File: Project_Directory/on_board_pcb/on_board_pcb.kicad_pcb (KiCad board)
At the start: 2 copper layers, 129.5 x 54.5 mm, 10 parts, among them U1 Teensy4.1

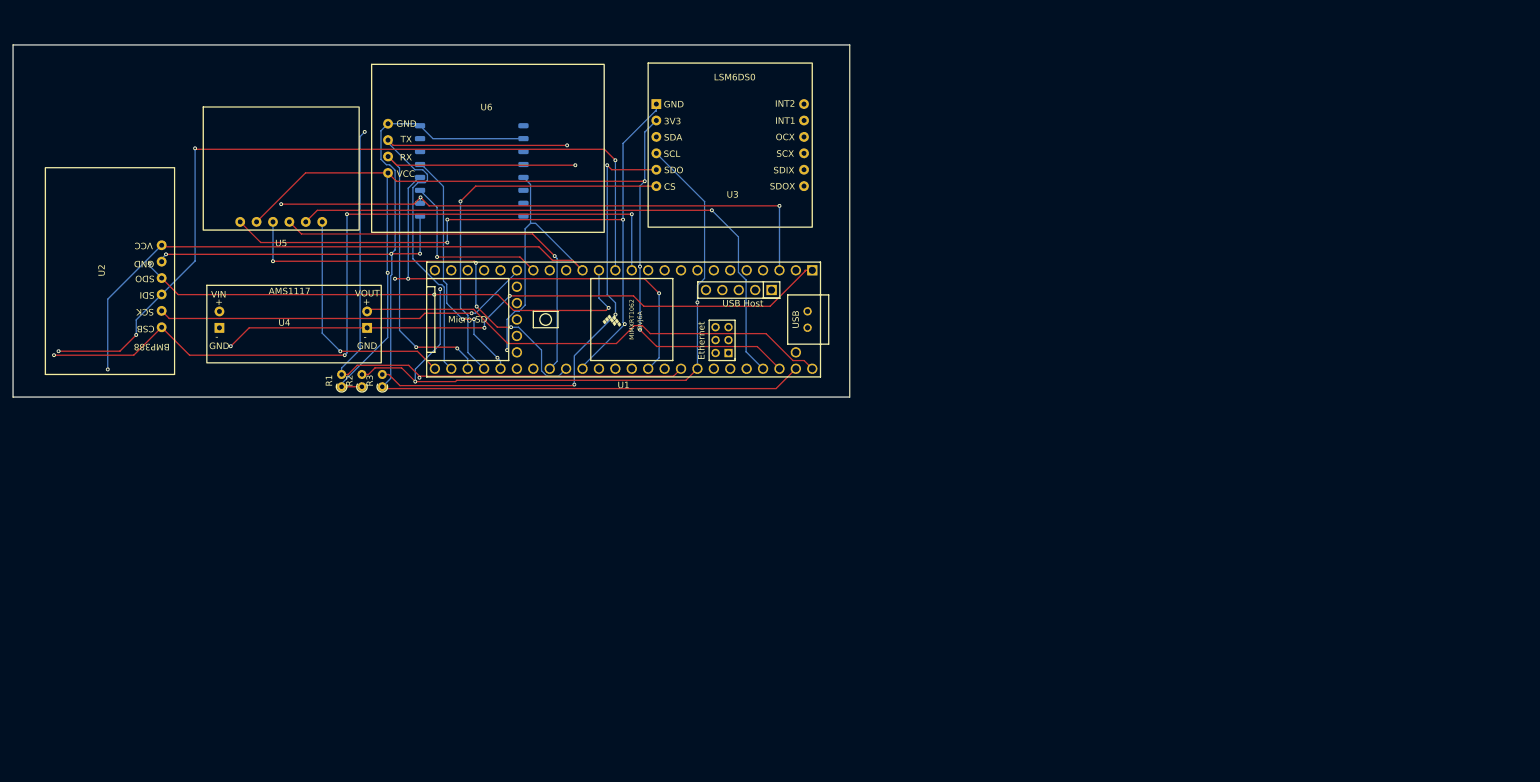
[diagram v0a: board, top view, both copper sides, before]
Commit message: preliminary pcb routing
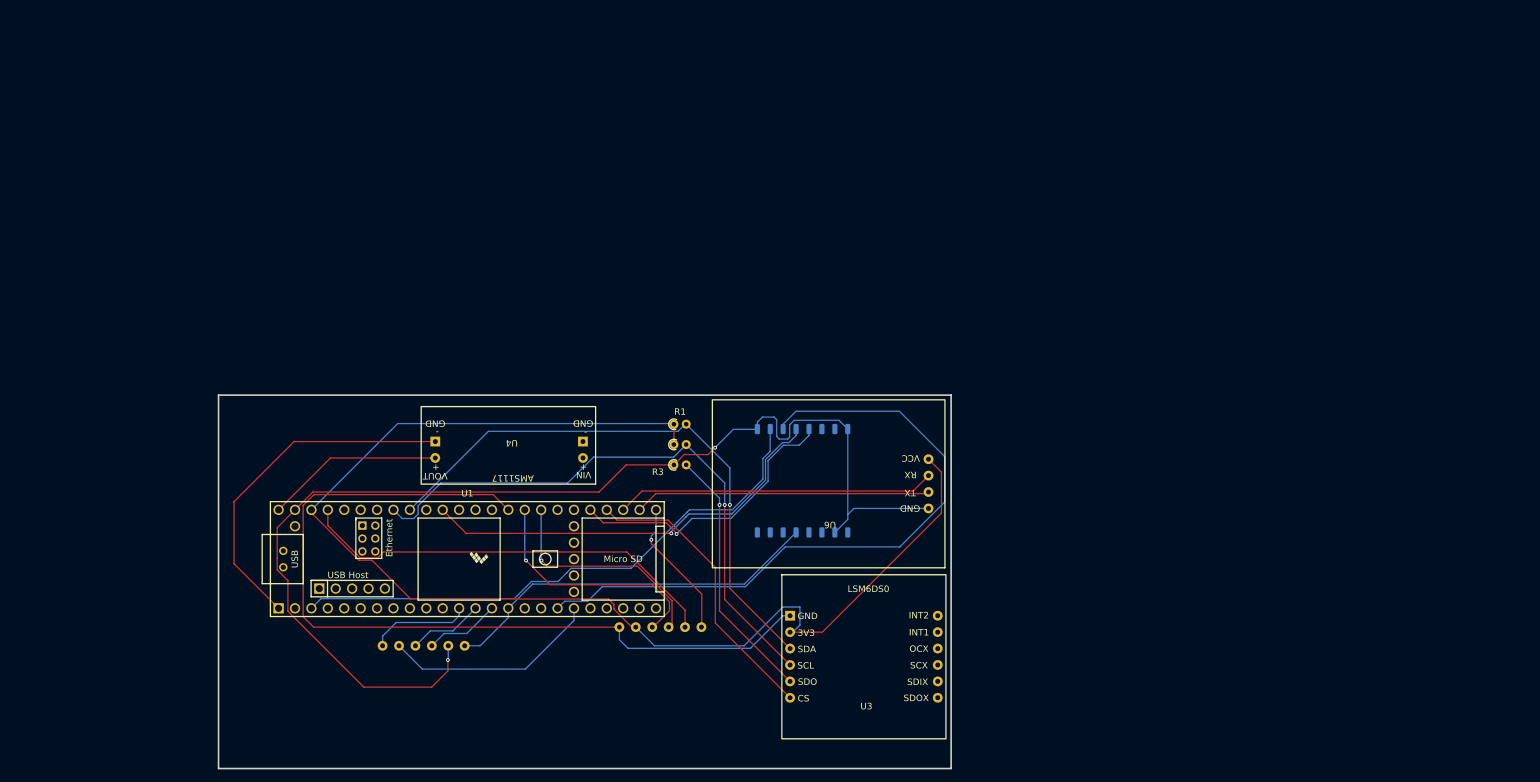
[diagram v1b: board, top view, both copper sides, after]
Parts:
- U2, U5: moved to B.Cu
- moved U3 81.9 mm to (174.7, 123.8)
- moved U5 80.5 mm to (143.2, 110.3)
- moved U2 77.7 mm to (112.9, 117.0), turned to 0 degrees
- moved U6 76.5 mm to (166.9, 95.7), turned to 180 degrees
- moved U7 70.8 mm to (165.7, 91.7), turned to -90 degrees
- moved R1 51.8 mm to (145.3, 82.7), turned to 0 degrees
- moved R2 49.1 mm to (145.3, 85.8), turned to 0 degrees
- moved R3 46.7 mm to (145.3, 89.0), turned to 0 degrees
- moved U1 44.3 mm to (113.3, 103.6), turned to 0 degrees
- moved U4 34.0 mm to (120.2, 87.7), turned to 180 degrees
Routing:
- net Net-(U1-11_MOSI_CTX1): track 128.6 -> 11.7 mm, vias 4 -> 0
- net Net-(U1-10_CS_MQSR): track 123.3 -> 16.3 mm, vias 4 -> 0
- net Net-(U1-26_A12_MOSI1): track 27.2 -> 103.3 mm, vias 1 -> 0
- net Net-(U2-VCC): track 129.6 -> 59.4 mm, vias 2 -> 0
- net Net-(U1-12_MISO_MQSL): track 80.9 -> 11.7 mm, vias 3 -> 0
- net Net-(U1-VIN): track 75.2 -> 27.6 mm
- net Net-(U1-GND-Pad1): track 96.9 -> 54.4 mm, vias 3 -> 0
- net Net-(U3-3V3): track 160.6 -> 197.5 mm, vias 4 -> 0
- net Net-(U3-SDO): track 75.5 -> 40.2 mm, vias 3 -> 1
- net Net-(U1-41_A17): track 65.0 -> 38.0 mm, vias 4 -> 1
- net Net-(U1-40_A16): track 61.3 -> 35.3 mm
- net Net-(U1-27_A13_SCK1): track 58.7 -> 33.6 mm, vias 1 -> 0
- net /Z: track 91.4 -> 66.5 mm, vias 1 -> 0
- net Net-(U1-34_RX8): track 71.0 -> 46.4 mm, vias 1 -> 0
- net Net-(U1-35_TX8): track 71.1 -> 49.5 mm, vias 3 -> 0
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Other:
- board size 129.5 x 54.5 mm -> 113.4 x 57.8 mm

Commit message: p1 board semifinal
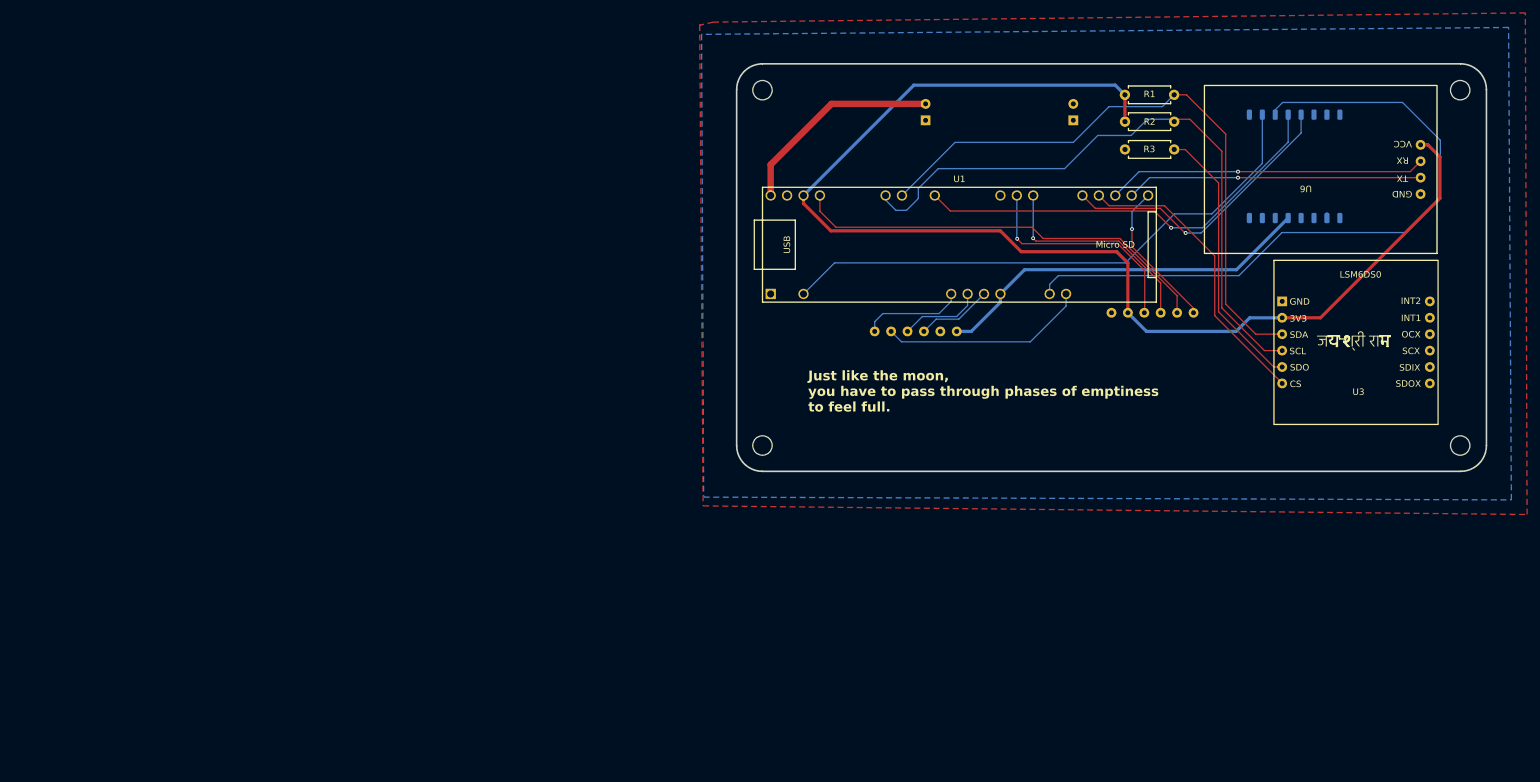
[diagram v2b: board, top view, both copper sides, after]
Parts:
- R1, R2, R3: footprint Resistor_THT:R_Axial_DIN0204_L3.6mm_D1.6mm_P1.90mm_Vertical -> Resistor_THT:R_Axial_DIN0207_L6.3mm_D2.5mm_P7.62mm_Horizontal
- U4: moved to B.Cu
- moved U4 93.3 mm to (196.1, 33.3)
- moved U5 90.4 mm to (219.4, 61.6)
- moved U7 90.4 mm to (241.9, 43.0)
- moved U3 90.4 mm to (250.9, 75.1)
- moved U6 90.4 mm to (243.1, 47.1)
- moved U1 90.4 mm to (189.5, 54.9)
- moved U2 90.4 mm to (189.1, 68.3)
- moved R1 86.4 mm to (215.1, 31.7)
- moved R2 85.9 mm to (215.1, 35.9)
- moved R3 85.2 mm to (215.1, 40.2)
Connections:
- U1 pad 1: Net-(U1-GND-Pad1) -> /GND
- U1 pad 34: /GND1 -> /GND
- U3 pad 1: /GND1 -> /GND
- U4 pad 4: Net-(U1-GND-Pad1) -> /GND
- U5 pad 1: /GND1 -> /GND
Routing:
- net /GND: track 179.8 -> 1.23 mm, vias 2 -> 0
- net /GND1: track 131.4 -> 0.00 mm
- net Net-(U1-GND-Pad1): track 54.4 -> 0.00 mm
- net Net-(U1-18_A4_SDA): track 89.7 -> 96.1 mm, vias 1 -> 0
- net Net-(U1-19_A5_SCL): track 92.1 -> 98.5 mm, vias 1 -> 0
- net Net-(U1-VIN): track 27.6 -> 32.6 mm
- net Net-(U3-3V3): track 197.5 -> 193.9 mm
- net Net-(U1-41_A17): track 38.0 -> 35.2 mm
- net Net-(U1-26_A12_MOSI1): track 103.3 -> 105.5 mm
- net Net-(U3-SDO): track 40.2 -> 42.2 mm, vias 1 -> 0
- net Net-(U1-27_A13_SCK1): track 33.6 -> 31.9 mm
- net Net-(U1-33_MCLK2): track 21.9 -> 23.3 mm
- net Net-(U1-40_A16): track 35.3 -> 34.2 mm
- net Net-(U1-11_MOSI_CTX1): track 11.7 -> 12.8 mm
- net Net-(U1-16_A2_RX4_SCL1): track 65.5 -> 66.5 mm
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- added copper zone on B.Cu, net /GND
- added copper zone on F.Cu, net /GND
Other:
- board size 113.4 x 57.8 mm -> 116.1 x 63.1 mm
- board text added: "Just like the moon, you have to pass through phases of emptiness to feel full."
- board text added: "The sky has no limits, neither should you."
